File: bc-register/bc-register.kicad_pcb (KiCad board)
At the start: 2 copper layers, 48.3 x 22.9 mm, 20 parts, among them J1 Conn_02x18_Odd_Even, U1 74LS377, U2 74LS245, U3 ULN2803A

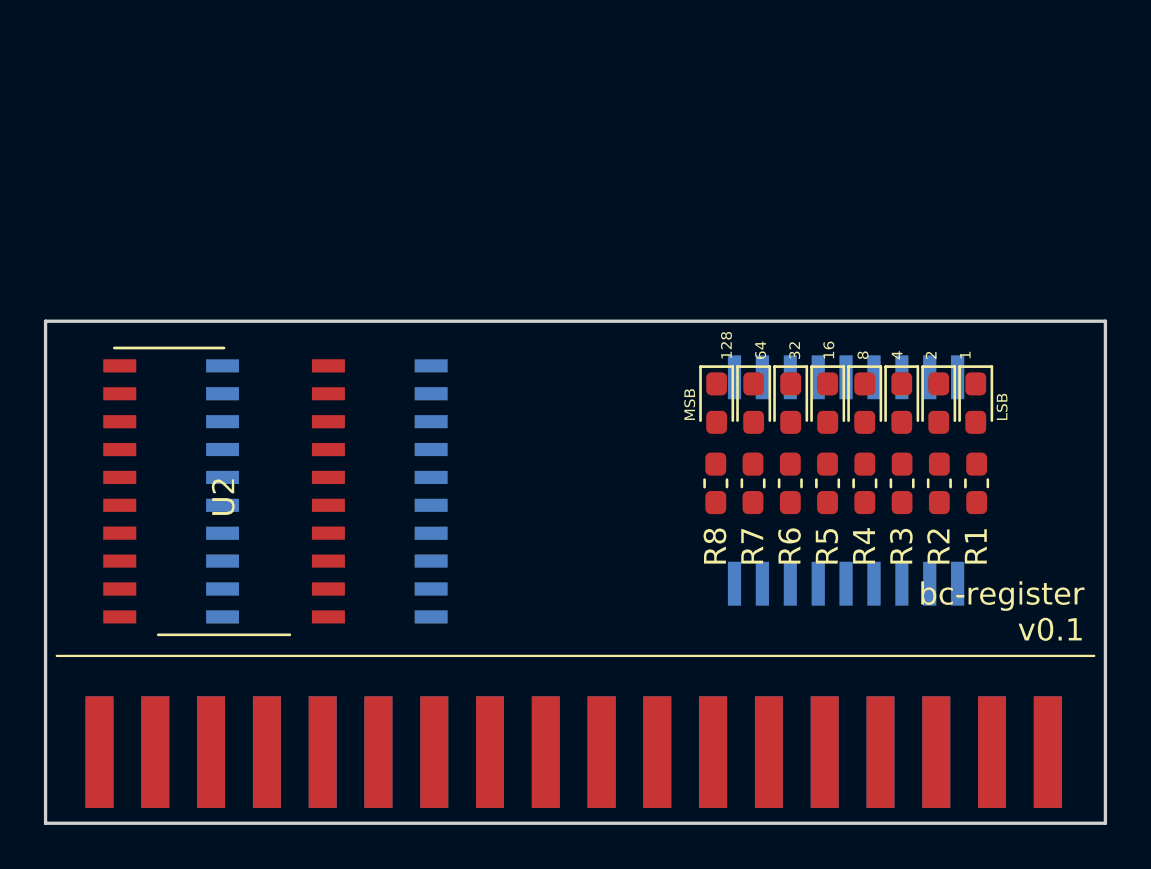
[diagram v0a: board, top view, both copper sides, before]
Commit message: trying out more things in bc-register
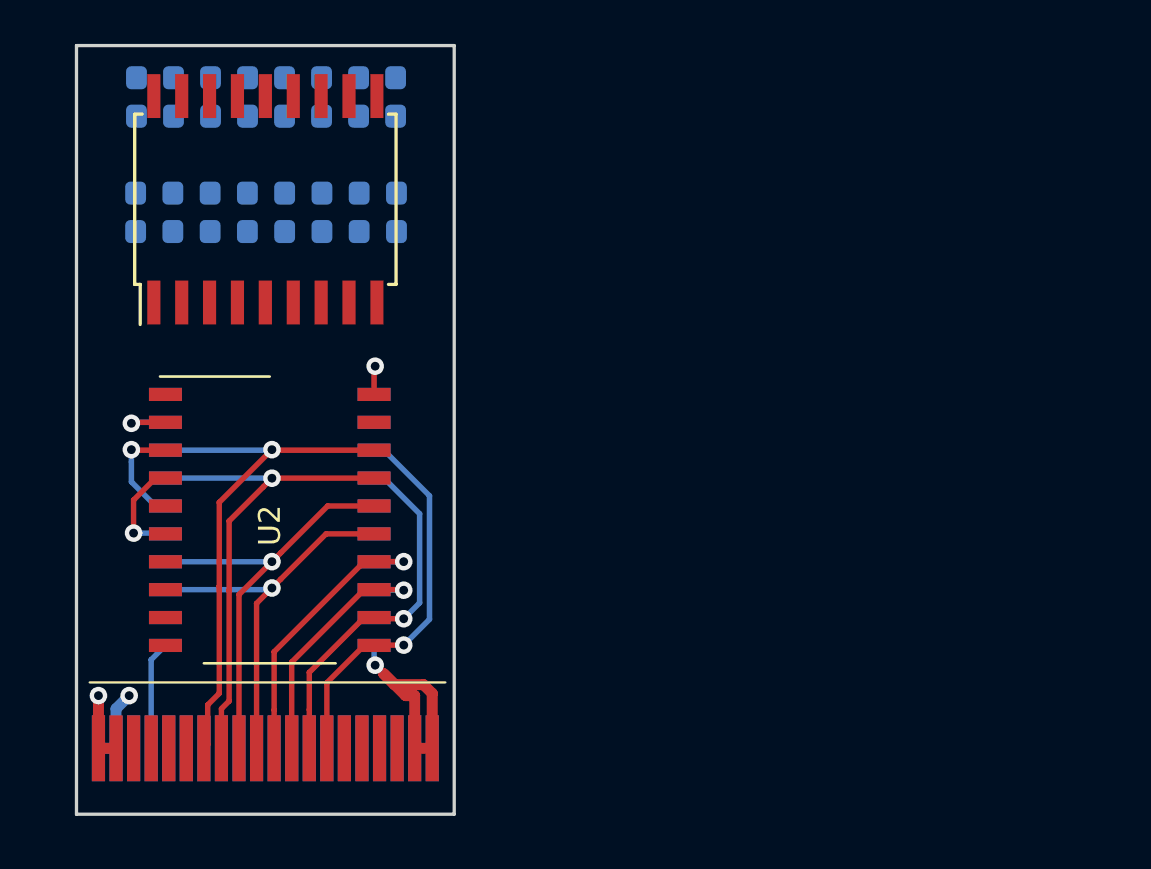
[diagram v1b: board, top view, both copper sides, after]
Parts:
- D1, D2, D3, D4, D5, D6, D7, D8, R1, R2, R3, R4, R5, R6, R7, R8: moved to B.Cu
- J1: value Conn_02x18_Odd_Even -> Conn_02x20_Odd_Even; footprint footprints:card-edge-2x18-100mils -> footprints:card-edge-2x20-800um
- U3: moved to F.Cu
- moved D1 40.7 mm to (143.3, 37.5)
- moved R1 40.2 mm to (143.3, 42.8)
- moved D2 37.5 mm to (145.0, 37.5)
- moved R2 37.0 mm to (145.0, 42.8)
- moved D3 34.4 mm to (146.7, 37.5)
- moved R3 33.8 mm to (146.7, 42.8)
- moved D4 31.4 mm to (148.4, 37.5)
- moved R4 30.7 mm to (148.4, 42.8)
- moved U3 29.4 mm to (149.2, 42.2)
- moved D5 28.4 mm to (150.1, 37.5)
- moved R5 27.6 mm to (150.1, 42.8)
- moved D6 25.5 mm to (151.8, 37.5)
- moved R6 24.6 mm to (151.8, 42.8)
- moved D7 22.8 mm to (153.4, 37.5)
- moved R7 21.8 mm to (153.5, 42.8)
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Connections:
- J1 pad 11: /BUS0 -> Net-(J1-Pad11)
- J1 pad 13: /BUS1 -> /BUS0
- J1 pad 15: /BUS2 -> /BUS1
- J1 pad 17: /BUS3 -> /BUS2
- J1 pad 19: /BUS4 -> /BUS3
- J1 pad 21: /BUS5 -> /BUS4
- J1 pad 23: /BUS6 -> /BUS5
- J1 pad 25: /BUS7 -> /BUS6
- J1 pad 27: Net-(J1-Pad27) -> /BUS7
- J1 pad 33: GND -> /CLK
- J1 pad 34: VCC -> Net-(J1-Pad34)
- J1 pad 35: GND -> /~IE
- J1 pad 36: VCC -> Net-(J1-Pad36)
- J1 pad 5: /~IE -> Net-(J1-Pad5)
- J1 pad 7: /CLK -> Net-(J1-Pad7)
- J1 pad 8: Net-(J1-Pad8) -> /CLK
- U1 pad 2: /RAW4 -> /RAW7
- U1 pad 3: /BUS4 -> /BUS7
- U1 pad 4: /BUS5 -> /BUS6
- U1 pad 5: /RAW5 -> /RAW6
- U1 pad 6: /RAW6 -> /RAW4
- U1 pad 7: /BUS6 -> /BUS4
- U1 pad 8: /BUS7 -> /BUS5
- U1 pad 9: /RAW7 -> /RAW5
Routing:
- net /BUS0: track 0.00 -> 24.4 mm, vias 0 -> 1
- net /BUS1: track 0.00 -> 22.8 mm, vias 0 -> 1
- net /BUS2: track 0.00 -> 19.7 mm, vias 0 -> 1
- net /BUS3: track 0.00 -> 18.1 mm, vias 0 -> 1
- net /BUS7: track 0.00 -> 17.9 mm, vias 0 -> 1
- net /BUS6: track 0.00 -> 16.6 mm, vias 0 -> 1
- net GND: track 0.00 -> 15.0 mm, vias 0 -> 2
- net /BUS4: track 0.00 -> 13.3 mm, vias 0 -> 1
- net /BUS5: track 0.00 -> 11.8 mm, vias 0 -> 1
- net /RAW1: track 0.00 -> 5.03 mm, vias 0 -> 1
- net /CLK: track 0.00 -> 4.95 mm
- net /RAW2: track 0.00 -> 4.83 mm, vias 0 -> 1
- net VCC: track 0.00 -> 4.59 mm, vias 0 -> 2
- net /RAW0: track 0.00 -> 3.14 mm, vias 0 -> 1
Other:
- board size 48.3 x 22.9 mm -> 17.2 x 35 mm
- board text added: "1"
- board text added: "128"
- board text added: "16"
- board text added: "2"
- board text added: "32"
- board text added: "4"
- board text added: "64"
- board text added: "8"
- board text removed: "128 64 32 16 8 4 2 1"
